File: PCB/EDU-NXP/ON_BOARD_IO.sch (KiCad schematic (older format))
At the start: 22 parts, among them SW2 SW_PUSH, SW3 SW_PUSH, SW4 SW_PUSH, SW5 SW_PUSH

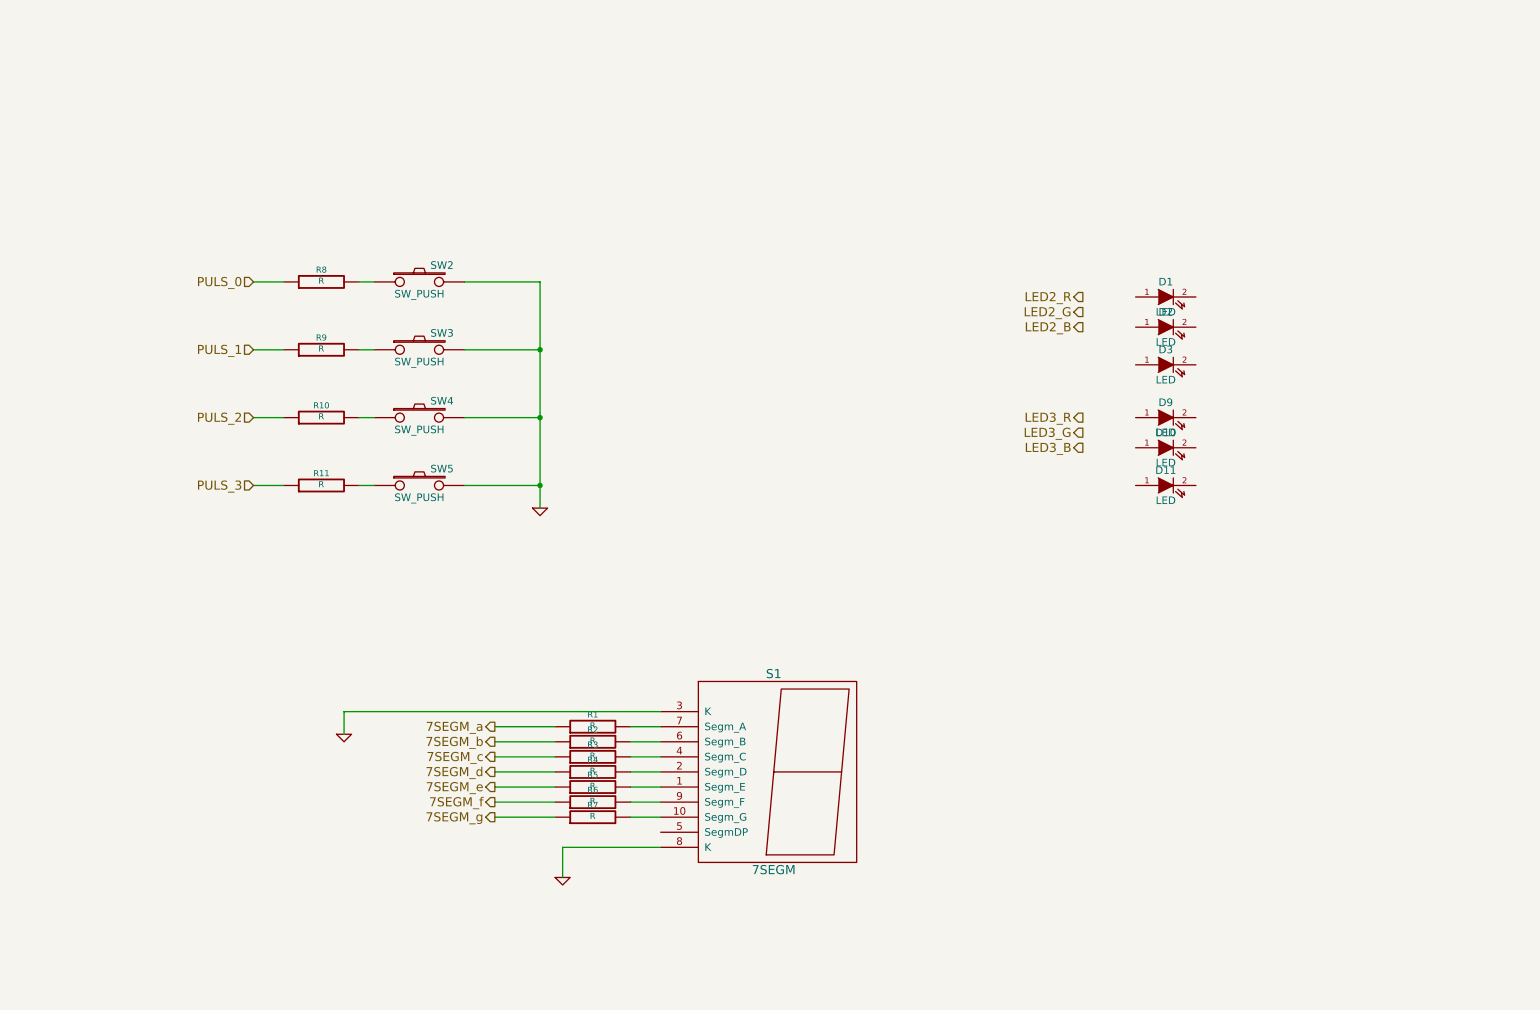
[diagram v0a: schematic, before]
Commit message: Versión con algunas mejoras
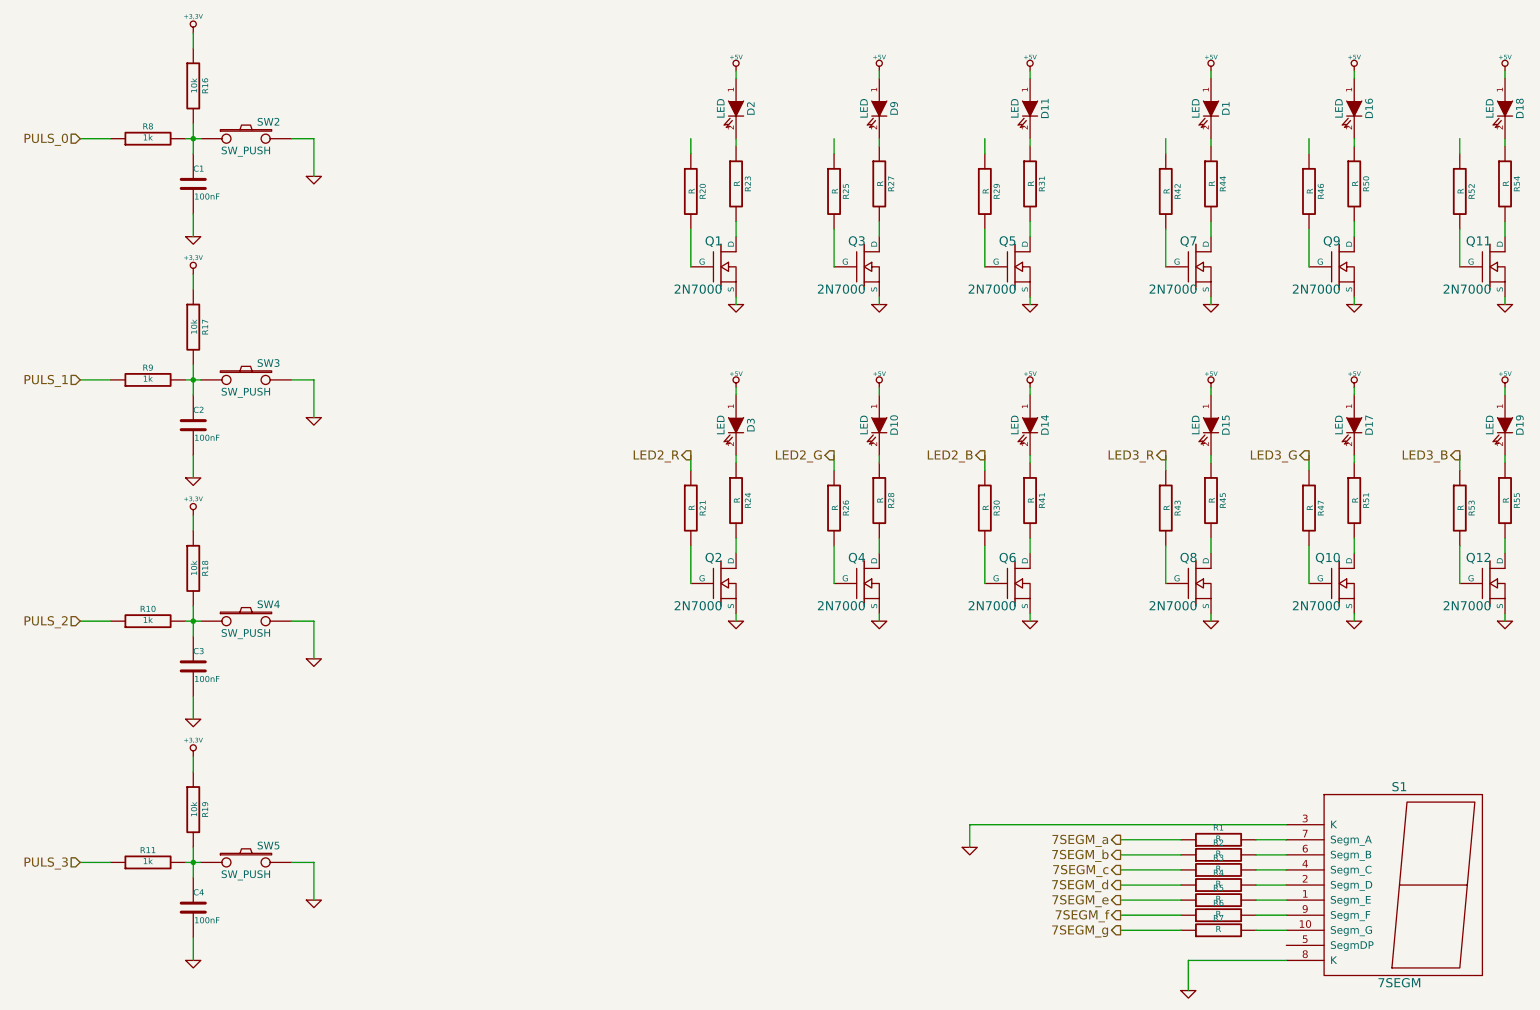
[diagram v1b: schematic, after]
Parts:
- added C1, C2, C3, C4: 100nF, ~, symbol C
- added D14, D15, D16, D17, D18, D19: LED, ~, symbol LED
- added Q1, Q10, Q11, Q12, Q2, Q3, Q4, Q5, Q6, Q7, Q8, Q9: 2N7000, ~, symbol MOSFET_N
- added R16, R17, R18, R19: 10k, ~, symbol R
- added R20, R21, R23, R24, R25, R26, R27, R28, R29, R30, R31, R41, R42, R43, R44, R45, R46, R47, R50, R51, R52, R53, R54, R55: R, ~, symbol R
- R10, R11, R8, R9: value R -> 1k
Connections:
- net labels added: +3,3V, +5V
- wire segments 31 -> 118
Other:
- moved on the sheet: D1, R1, R2, R3, R4, R5, R6, R7, R8, S1, SW2
